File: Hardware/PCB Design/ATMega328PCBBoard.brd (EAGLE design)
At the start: 40.3 x 19.1 mm, 14 parts

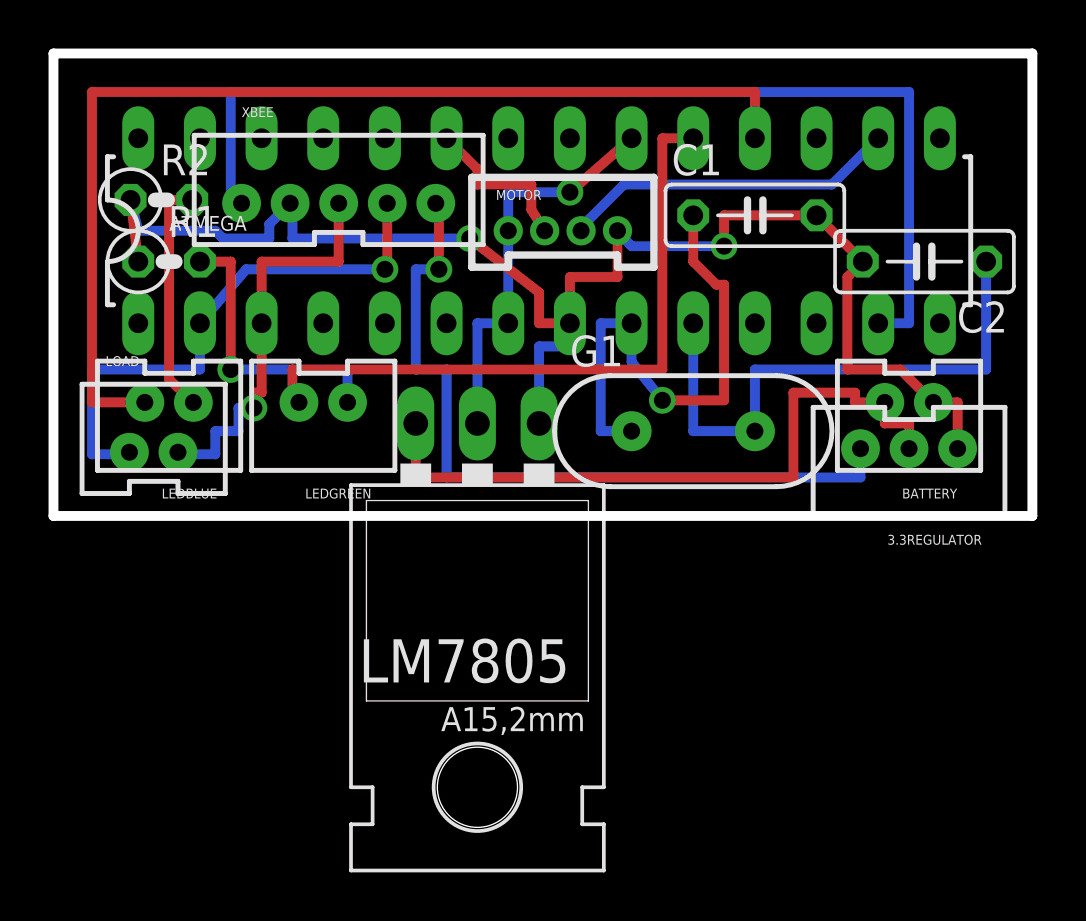
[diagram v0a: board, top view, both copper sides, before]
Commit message: final board design
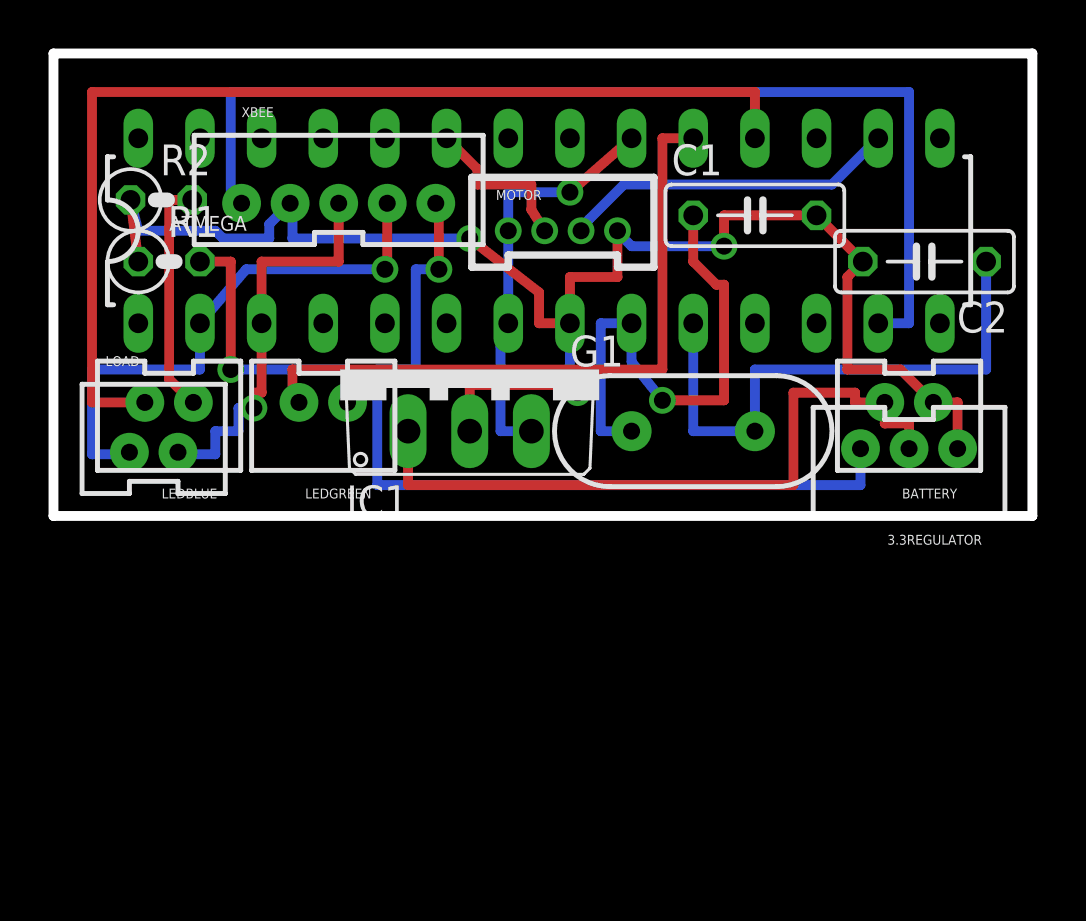
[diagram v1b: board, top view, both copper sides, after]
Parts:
- removed LM7805: V_REG_LD1117VXX, SparkFun-PowerIC:78XXL
- added IC1: 7805TV, linear:TO220V
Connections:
- net GND: now also IC1.2; no longer LM7805.IN
- net N$4: now also IC1.1; no longer LM7805.OUT
- net VCC: now also IC1.3; no longer LM7805.GND
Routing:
- net GND: track 61.6 -> 66.0 mm, vias 2 -> 3
- net 3VCC: track 31.9 -> 35.7 mm
- net N$4: track 28.3 -> 29.0 mm
- net VCC: track 16.7 -> 17.3 mm
